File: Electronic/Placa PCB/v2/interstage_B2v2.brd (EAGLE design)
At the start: 82.5 x 29 mm, 7 parts, among them P1 0532610271, Q1 PMV16XNR, U1 MCP9808T-E/MS, U3 MCP9808T-E/MS

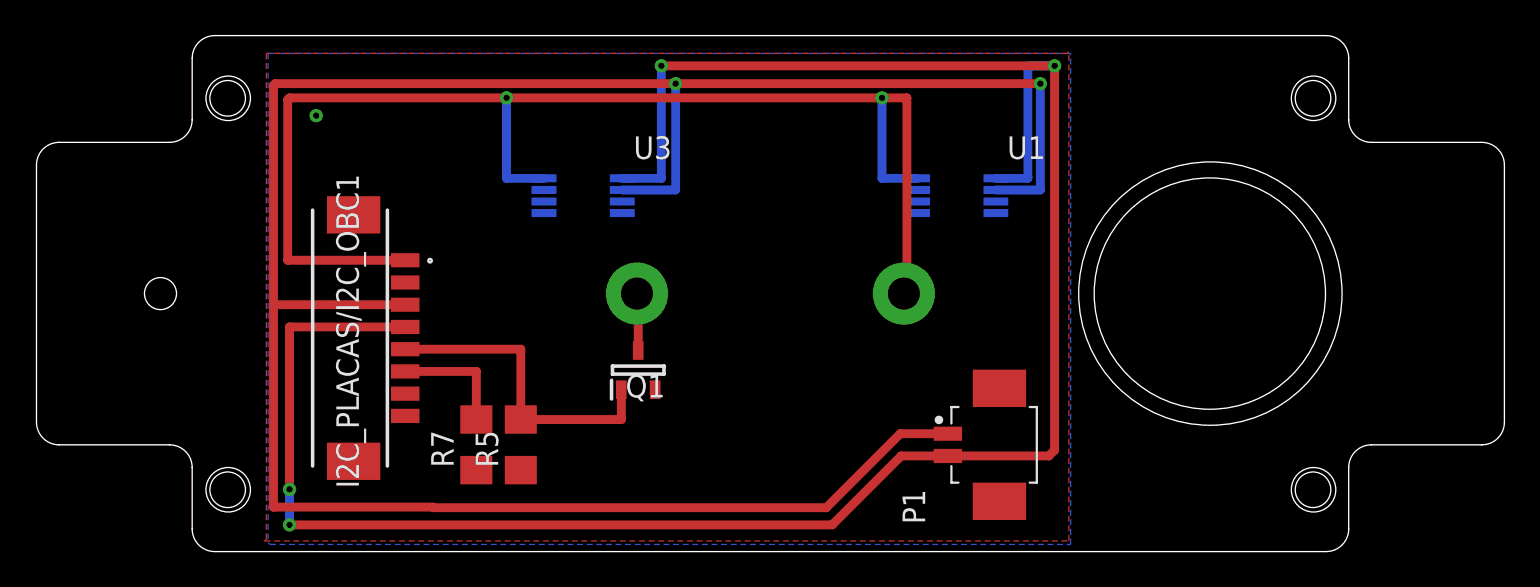
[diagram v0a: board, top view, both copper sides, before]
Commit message: Placas PCB
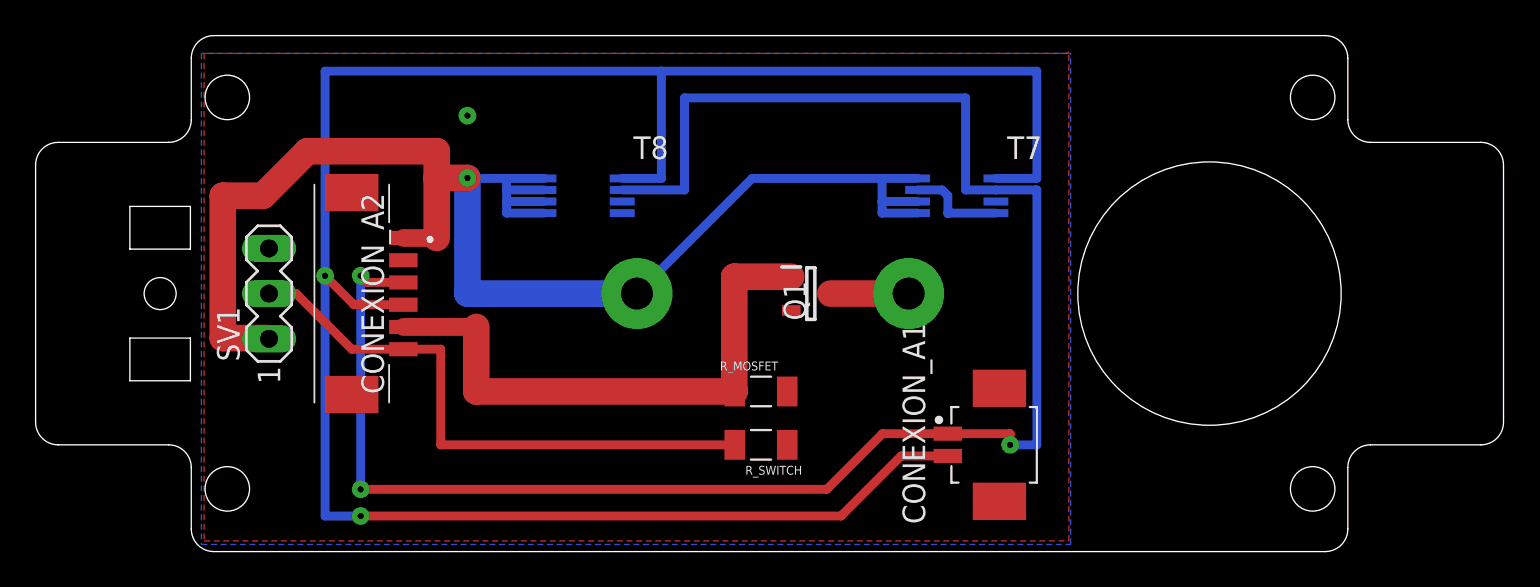
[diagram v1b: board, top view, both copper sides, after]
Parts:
- removed I2C_PLACAS/I2C_OBC1: 53261-0871, SamacSys_Parts:53261-0871
- removed R5, R7: 330 Ohm, rcl:R1206
- added CONEXION_A2: 53261-7006, SamacSys_Parts:532617006
- added R_MOSFET, R_SWITCH: ERA-8AEB331V, resistor_330_smd:RESC3216X70N
- added SV1: (no value), con-lstb:MA03-1
- moved Q1 10.6 mm to (34.8, 14.5), turned to 0 degrees
- renumbered P1 to CONEXION_A1, U1 to T7, U3 to T8
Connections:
- net MOSFET renamed NICROMO
- removed net N$1: R7.1
- net GND: now also CONEXION_A2.2, R_MOSFET.2, R_SWITCH.1, T7.7; no longer I2C_PLACAS/I2C_OBC1.2, R5.1
- net INT0: now also CONEXION_A2.6, R_SWITCH.2, SV1.2; no longer I2C_PLACAS/I2C_OBC1.6, R7.2
- net OC1A: now also CONEXION_A2.5, R_MOSFET.1; no longer I2C_PLACAS/I2C_OBC1.5, R5.2
- net SCL: now also CONEXION_A2.3; no longer I2C_PLACAS/I2C_OBC1.3
- net SDA: now also CONEXION_A2.4; no longer I2C_PLACAS/I2C_OBC1.4
- net VCC: now also CONEXION_A2.1, SV1.1, T7.5, T7.6, T8.5, T8.6, T8.7; no longer I2C_PLACAS/I2C_OBC1.1
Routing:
- net SCL: track 131.3 -> 102.4 mm, vias 2 -> 3
- net INT0: track 6.70 -> 32.8 mm
- net OC1A: track 17.8 -> 31.9 mm
- net VCC: track 74.7 -> 85.2 mm, vias 3 -> 2
- net GND: track 0.00 -> 5.54 mm
- net NICROMO: track 3.23 -> 4.40 mm
- net SDA: track 124.1 -> 123.0 mm, vias 4 -> 2
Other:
- outline, holes or cut-outs redrawn
